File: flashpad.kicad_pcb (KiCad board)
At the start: 2 copper layers, 61.2 x 65.3 mm, 23 parts, among them U1 ATmega328P-PU, U2 ATmega32A-PU

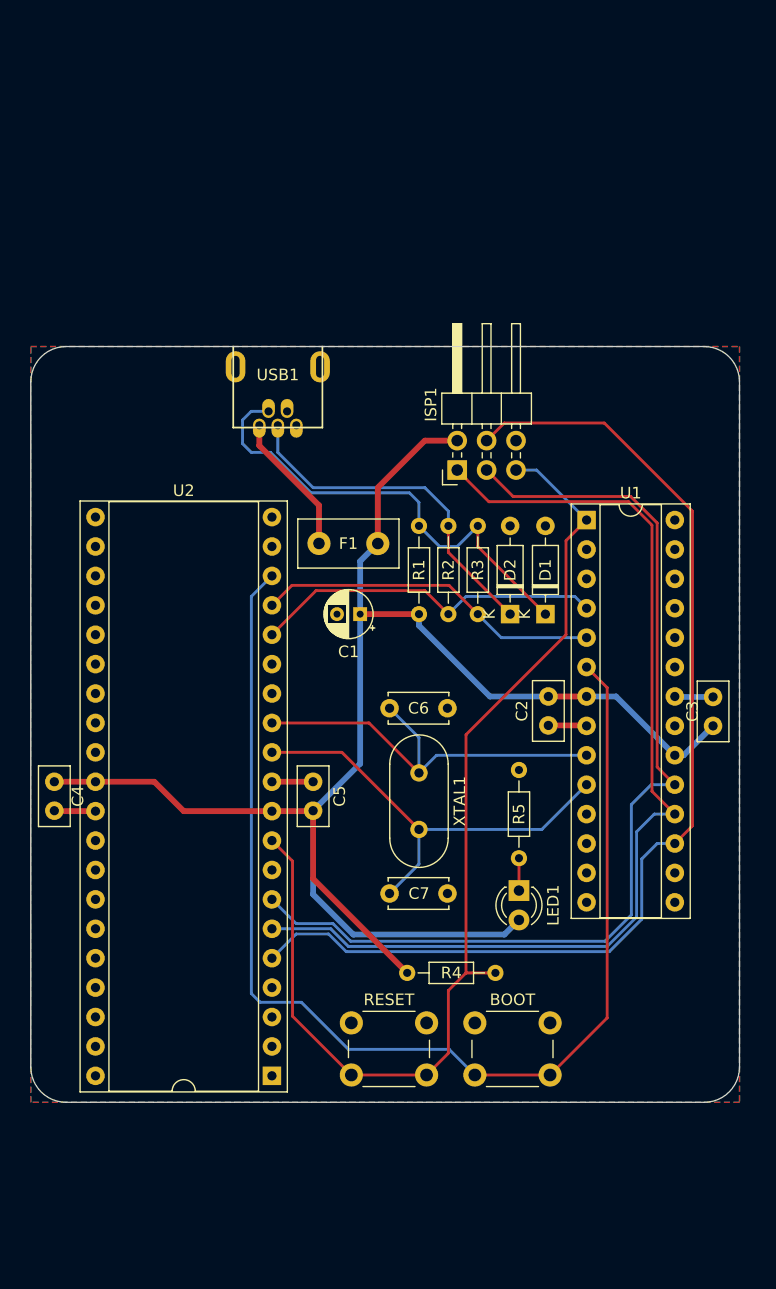
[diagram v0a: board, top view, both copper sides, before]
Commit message: rev2
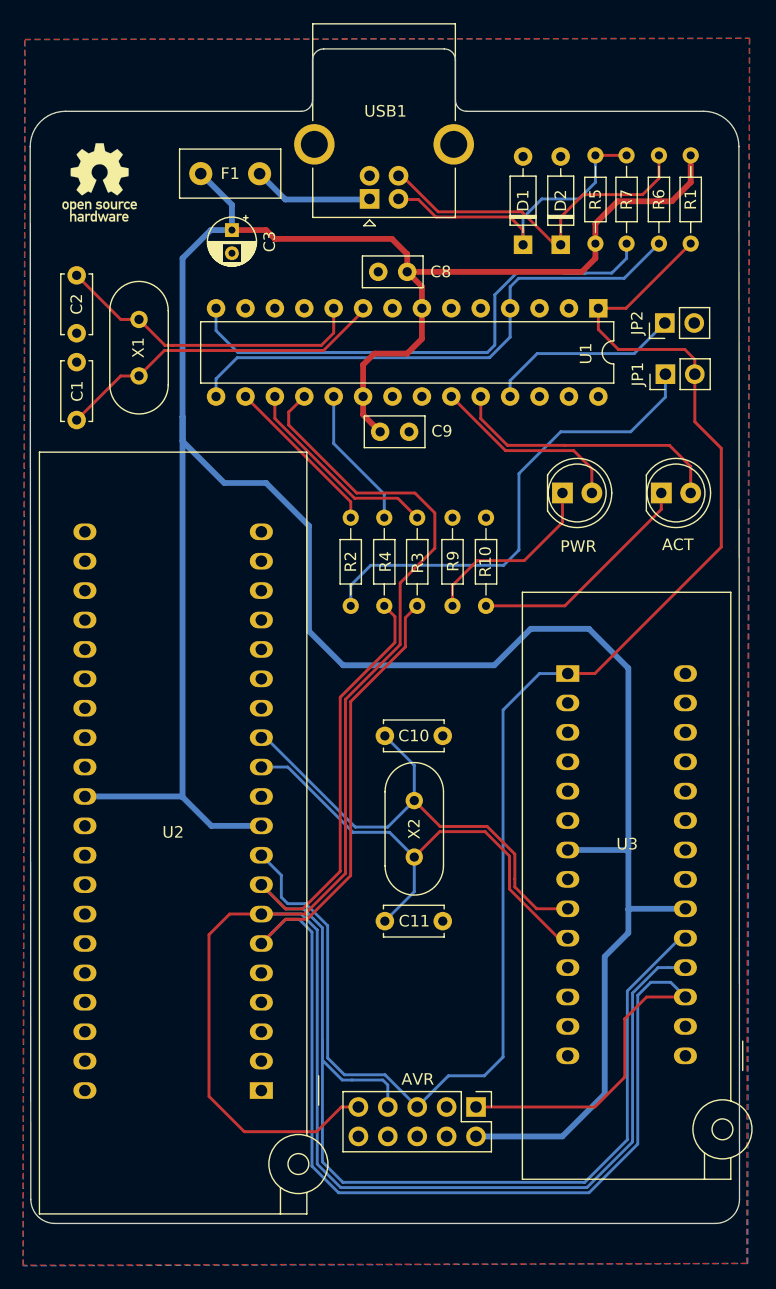
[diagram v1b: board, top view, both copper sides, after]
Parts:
- removed BOOT: BOOT, Button_Switch_THT:SW_PUSH_6mm
- removed the C3 at (155.2, 110.2)
- removed C4, C5: 100n, Capacitor_THT:C_Disc_D5.0mm_W2.5mm_P2.50mm
- removed C6, C7: 22p, Capacitor_THT:C_Disc_D5.0mm_W2.5mm_P5.00mm
- removed ISP1: AVR-ISP-6, Connector_PinHeader_2.54mm:PinHeader_2x03_P2.54mm_Horizontal
- removed LED1: LED, LED_THT:LED_D3.0mm
- removed the R5 at (138.4, 114.0)
- removed RESET: RESET, Button_Switch_THT:SW_PUSH_6mm
- removed XTAL1: Crystal, Crystal:Crystal_HC49-4H_Vertical
- added ACT: LED, LED_THT:LED_D5.0mm, F.Cu at (150.7, 90.1)
- added AVR: AVR-ISP-10, Connector_PinHeader_2.54mm:PinHeader_2x05_P2.54mm_Vertical, F.Cu at (134.7, 143.2)
- added C1: 22p, Capacitor_THT:C_Disc_D5.0mm_W2.5mm_P5.00mm, F.Cu at (100.2, 83.8)
- added C10: 22p, Capacitor_THT:C_Disc_D5.0mm_W2.5mm_P5.00mm, F.Cu at (126.8, 111.1)
- added C11: 22p, Capacitor_THT:C_Disc_D5.0mm_W2.5mm_P5.00mm, F.Cu at (126.8, 127.1)
- added C8: 100n, Capacitor_THT:C_Disc_D5.0mm_W2.5mm_P2.50mm, F.Cu at (128.8, 71.0)
- added C9: 100n, Capacitor_THT:C_Disc_D5.0mm_W2.5mm_P2.50mm, F.Cu at (126.4, 84.8)
- added G***: LOGO, custom_parts:elmo, B.Cu at (102.3, 63.4)
- added G***: LOGO, custom_parts:oshw, F.Cu at (102.2, 63.3)
- added JP1: SelfProg, Connector_PinHeader_2.54mm:PinHeader_1x02_P2.54mm_Vertical, F.Cu at (151.1, 79.9)
- added JP2: SlowSCK, Connector_PinHeader_2.54mm:PinHeader_1x02_P2.54mm_Vertical, F.Cu at (151.0, 75.4)
- added PWR: LED, LED_THT:LED_D5.0mm, F.Cu at (142.2, 90.1)
- added R1: 10k, Resistor_THT:R_Axial_DIN0204_L3.6mm_D1.6mm_P7.62mm_Horizontal, F.Cu at (153.3, 61.0)
- added R10: 1.5K, Resistor_THT:R_Axial_DIN0204_L3.6mm_D1.6mm_P7.62mm_Horizontal, F.Cu at (135.6, 92.3)
- added R2: 270r, Resistor_THT:R_Axial_DIN0204_L3.6mm_D1.6mm_P7.62mm_Horizontal, F.Cu at (123.9, 92.3)
- added R3: 270r, Resistor_THT:R_Axial_DIN0204_L3.6mm_D1.6mm_P7.62mm_Horizontal, F.Cu at (129.6, 92.3)
- added R9: 1.5K, Resistor_THT:R_Axial_DIN0204_L3.6mm_D1.6mm_P7.62mm_Horizontal, F.Cu at (132.7, 92.3)
- added U1: ATmega8A-PU, Package_DIP:DIP-28_W7.62mm, F.Cu at (145.3, 74.2)
- added X1: 12Mhz, Crystal:Crystal_HC49-4H_Vertical, F.Cu at (105.6, 80.0)
- added X2: 16Mhz, Crystal:Crystal_HC49-4H_Vertical, F.Cu at (129.4, 116.7)
- C2: value 100n -> 22p; footprint Capacitor_THT:C_Disc_D5.0mm_W2.5mm_P2.50mm -> Capacitor_THT:C_Disc_D5.0mm_W2.5mm_P5.00mm
- R4: value 1.5K -> 270r
- R5: renamed from R1; value 1.5K -> 2.2k
- U2: footprint Package_DIP:DIP-40_W15.24mm_Socket -> Socket:DIP_Socket-40_W11.9_W12.7_W15.24_W17.78_W18.5_3M_240-1280-00-0602J
- U3: renamed from U1; footprint Package_DIP:DIP-28_W7.62mm_Socket -> custom_parts:DIP_Socket-28_flipped
- USB1: value USB_B_Mini -> USB_B; footprint custom_parts:USB_Mini -> Connector_USB:USB_B_OST_USB-B1HSxx_Horizontal
- moved C2 54.6 mm to (100.2, 71.3)
- moved U3 47.1 mm to (152.8, 138.7), turned to 180 degrees
- moved R4 40.5 mm to (126.8, 92.3), turned to 270 degrees
- moved R6 36.8 mm to (150.5, 61.0)
- moved R5 35.4 mm to (145.0, 68.6)
- moved F1 35.4 mm to (110.9, 62.5), turned to 0 degrees
- moved C3 35.0 mm to (113.6, 67.4), turned to 270 degrees
- moved R7 34.5 mm to (147.7, 61.0)
- moved D2 32.2 mm to (142.0, 68.7)
- moved D1 32.0 mm to (138.8, 68.7)
- moved USB1 15.0 mm to (125.5, 64.7), turned to 90 degrees
- moved U2 1.56 mm to (116.2, 141.7)
- renumbered C1 to C3, R2 to R6, R3 to R7
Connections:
- net XTAL1 renamed XTAL2_1
- net XTAL2 renamed XTAL2_2
- C2 pad 1: +5V -> XTAL1_2
- R4 pad 1: RESET -> Net-(R4-Pad1)
- R4 pad 2: +5V -> SCK
- U2 pad 16: D+ -> Net-(U2-Pad16)
- U2 pad 17: D- -> Net-(U2-Pad17)
- U2 pad 18: BOOT -> Net-(U2-Pad18)
- U2 pad 5: MOSI -> Net-(U2-Pad5)
- U2 pad 6: MISO -> MOSI
- U2 pad 7: SCK -> MISO
- U2 pad 8: Net-(U2-Pad8) -> SCK
- U3 pad 4: D+ -> Net-(U3-Pad4)
- U3 pad 5: D- -> Net-(U3-Pad5)
- U3 pad 6: BOOT -> Net-(U3-Pad6)
- USB1 pad 4: Net-(USB1-Pad4) -> GND
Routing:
- net +5V: track 143.7 -> 259.3 mm
- net BOOT: track 103.5 -> 0.00 mm
- net MISO: track 89.0 -> 169.8 mm
- net Net-(JP1-Pad1): track 0.00 -> 41.5 mm
- net MOSI: track 94.1 -> 135.5 mm
- net RESET: track 93.7 -> 132.8 mm
- net SCK: track 87.3 -> 120.0 mm
- net XTAL1_1: track 0.00 -> 28.9 mm
- net XTAL1_2: track 0.00 -> 27.3 mm
- net LED2: track 0.00 -> 24.0 mm
- net Net-(LED2-Pad1): track 0.00 -> 20.0 mm
- net Net-(R3-Pad1): track 0.00 -> 17.7 mm
- net D-: track 29.8 -> 47.1 mm
- net D+: track 30.6 -> 47.7 mm
- net LED1: track 0.00 -> 16.8 mm
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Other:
- board size 61.2 x 65.3 mm -> 61.3 x 101.4 mm
- rule pad_to_mask_clearance: 0.05 -> 0
- board text added: "USBasp MultiPad by kb-elmo github.com/kb_elmo"
